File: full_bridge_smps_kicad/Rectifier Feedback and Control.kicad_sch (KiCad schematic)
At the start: 32 parts, among them J6 Conn_01x04_Male, J7 Conn_01x02_Male, U1 MSP430F2012IPW, U1 TPS3809I50DBV, U3 OPA333AID

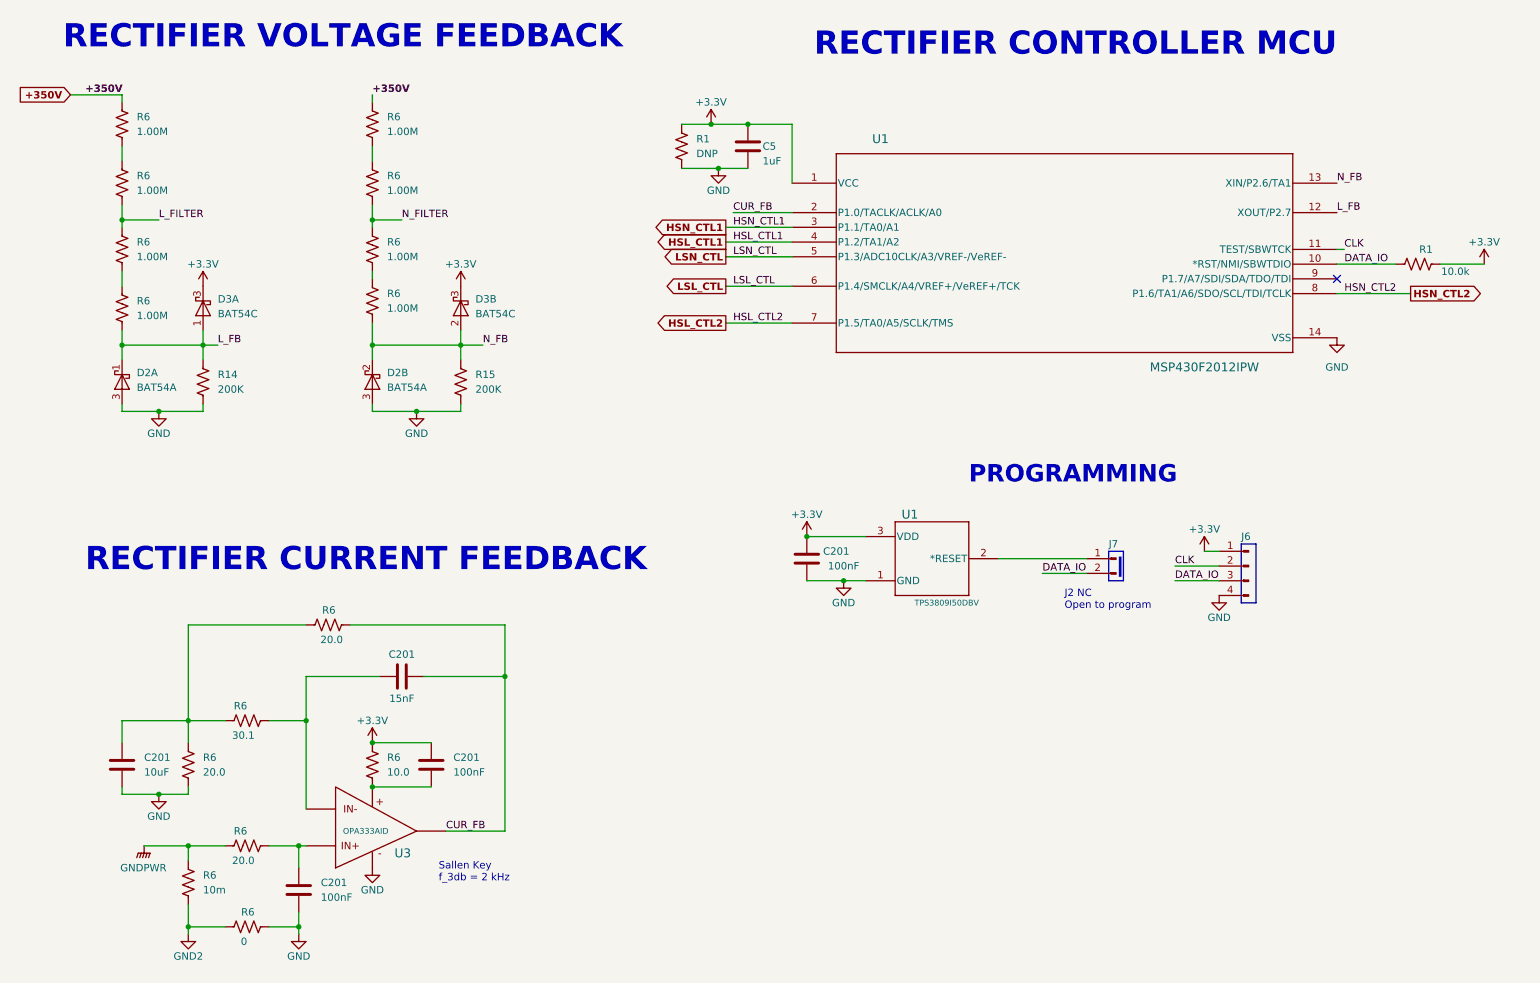
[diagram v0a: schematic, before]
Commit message: A bit of refactoring, saving work for the day
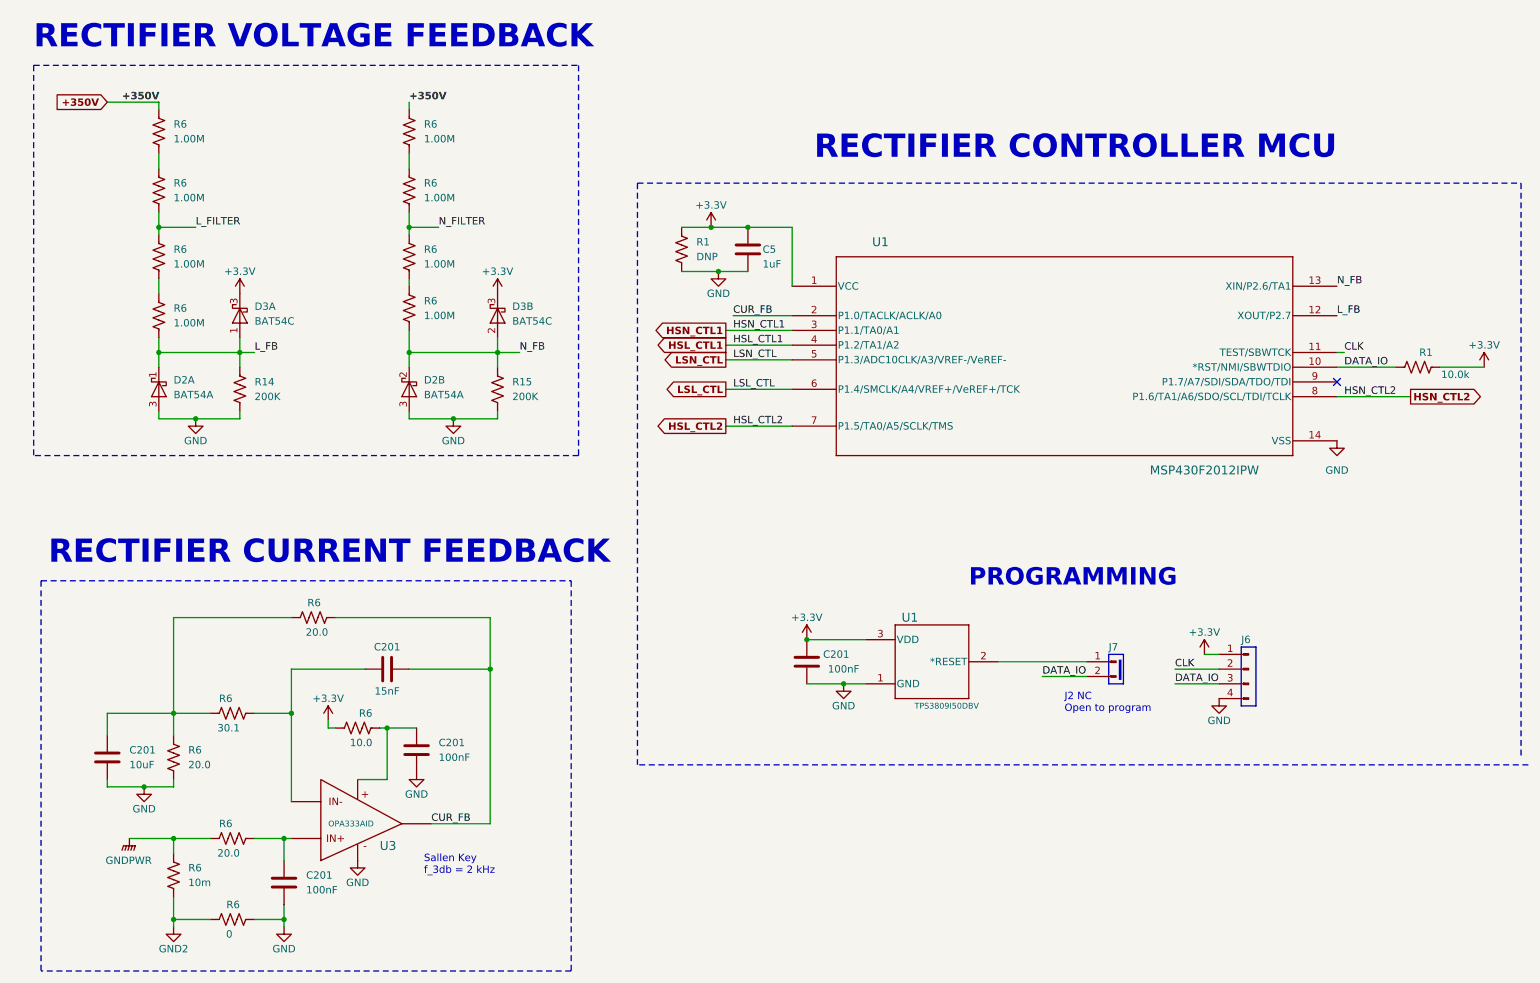
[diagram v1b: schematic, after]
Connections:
- net +3V3: no longer C201.1
- net GND: now also C201.2
- net V+: now also C201.1; no longer C201.2
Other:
- moved on the sheet: C201, C5, D2A, D2B, D3A, D3B, J6, J7, R1, R14, R15, R6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
